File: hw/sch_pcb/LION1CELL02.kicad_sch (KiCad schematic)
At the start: 82 parts, among them IC1 BQ294602DRVR, J1 CONN1_1, J10 JUMP_2x1, J11 JUMP_2x1, J12 JUMP_2x1, J13 JUMP_2x1, J2 CONN1_1, J3 Jack-DC, J4 JUMP_2x1, J5 JUMP_2x1, J6 JUMP_2x1, J7 JUMP_2x1, J8 JUMP2_2x1, J9 Conn_02x03_Odd_Even, M1 HOLE M3, M2 HOLE M3, M3 HOLE, M4 HOLE, Q1 IRLML6244, SW1 SW_PUSH, U1 BQ24103, U2 SN74HC164D, U3 BQ34Z100

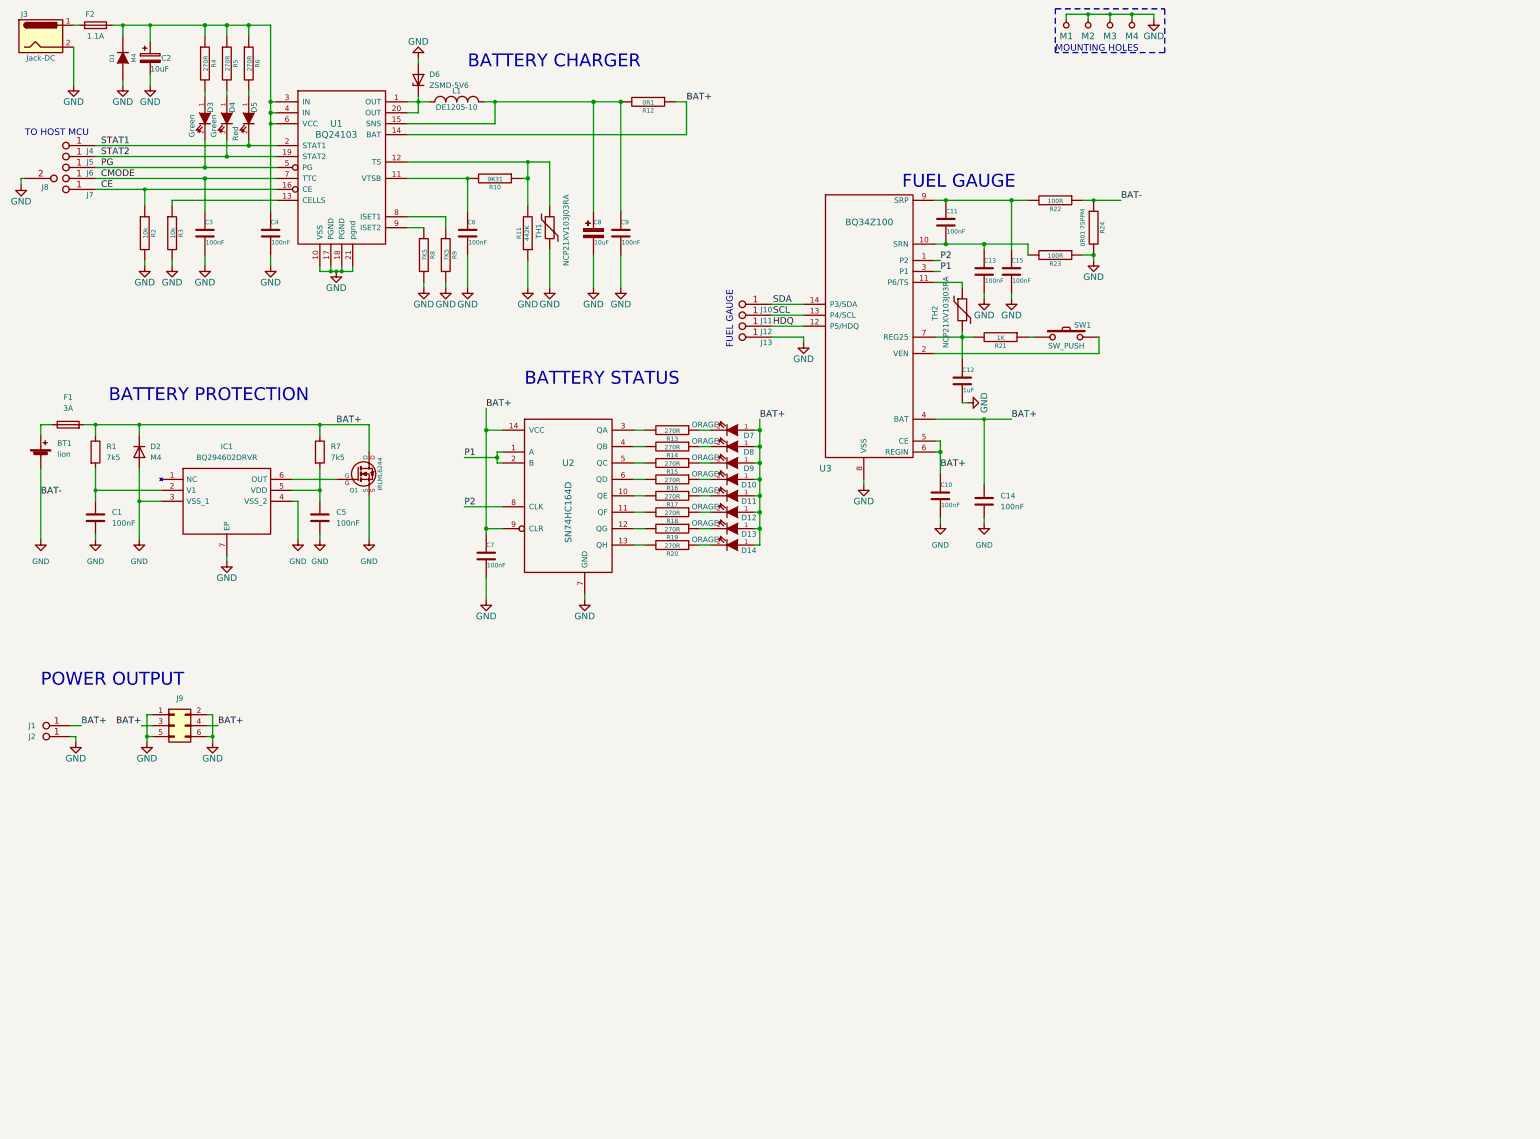
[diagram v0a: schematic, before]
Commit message: Update schematics
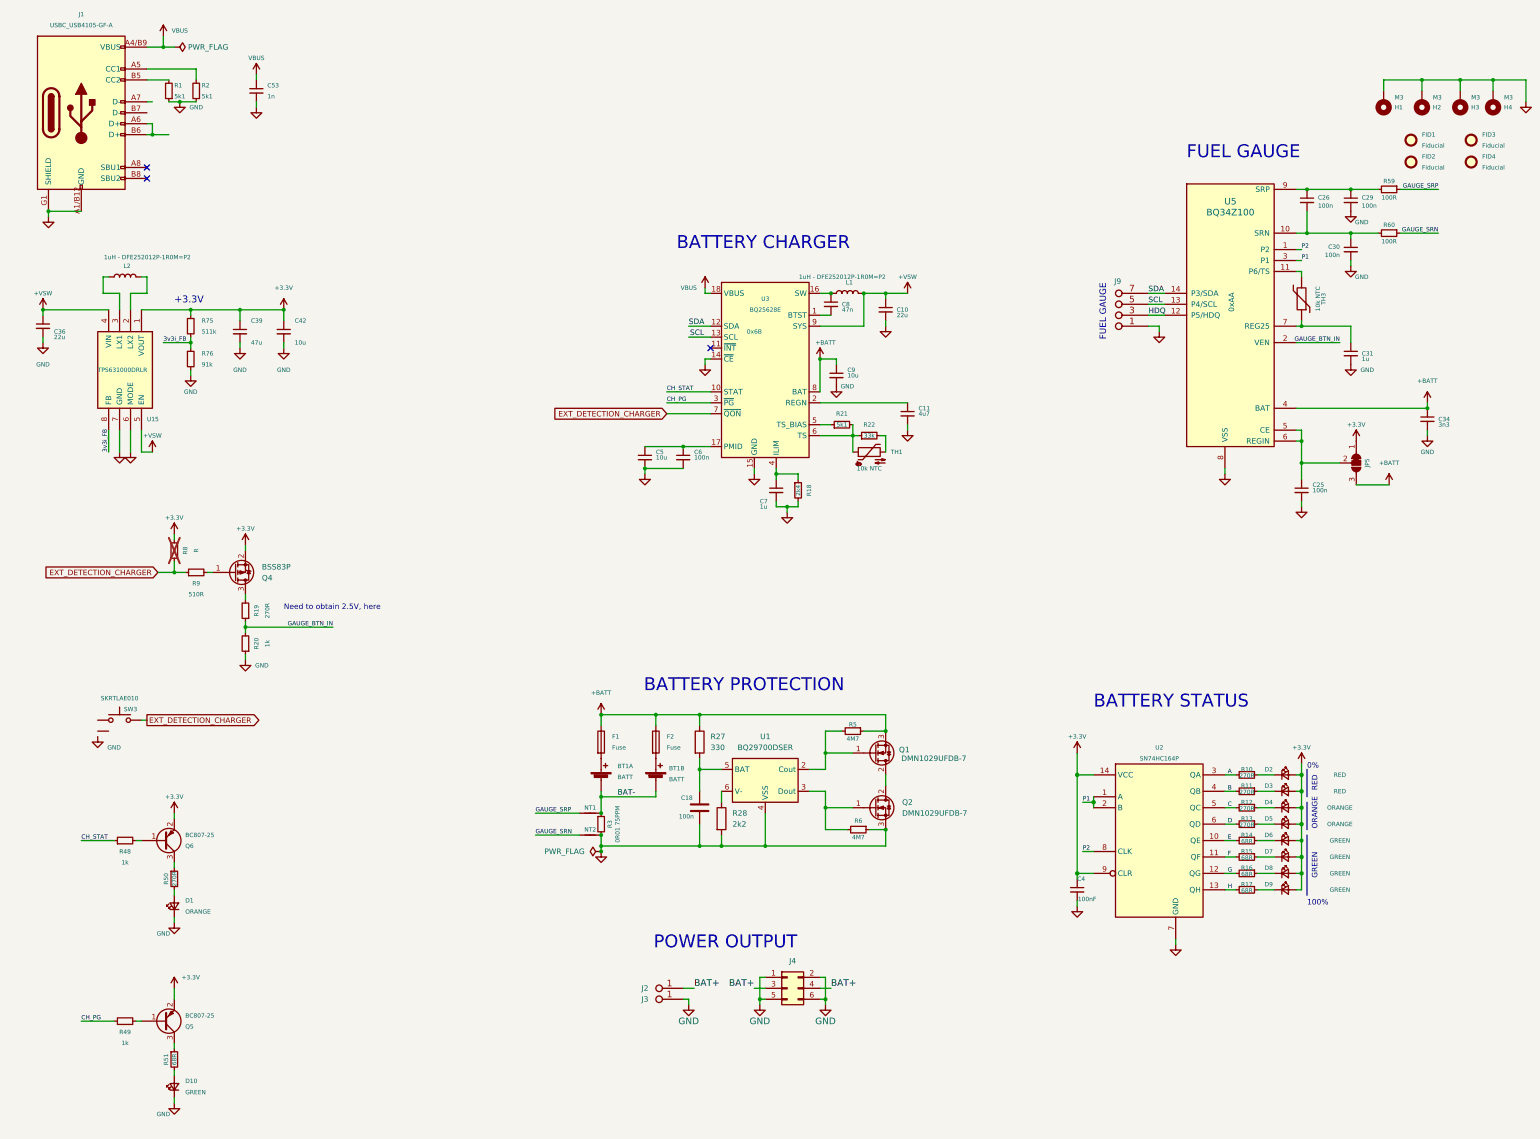
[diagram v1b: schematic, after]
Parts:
- removed BT1: lion, symbol Device:Battery_Cell
- removed C1, C14, C5: 100nF, Mlab_C:SMD-0805, symbol Device:C
- removed C10, C11, C13, C3, C4, C6, C7, C9: 100nF, Mlab_C:SMD-0805, symbol LION2CELL01D-rescue:C-RESCUE-LION2CELL01C
- removed C12: 1uF, Mlab_C:SMD-0805, symbol LION2CELL01D-rescue:C-RESCUE-LION2CELL01C
- removed C15: 100nF, Mlab_R:SMD-0805, symbol LION2CELL01D-rescue:C-RESCUE-LION2CELL01C
- removed C2: 10uF, Mlab_C:TantalC_SizeD_Reflow, symbol Device:C_Polarized
- removed C8: 10uF, Mlab_C:TantalC_SizeD_Reflow, symbol LION2CELL01D-rescue:CP2
- removed D1: M4, Mlab_D:SMA_Standard, symbol LION2CELL01D-rescue:DIODE
- removed D10, D11, D12, D13, D14, D7, D8, D9: ORAGE, Mlab_D:LED_1206, symbol LION2CELL01D-rescue:LED-RESCUE-LION2CELL01C
- removed D2: M4, symbol Device:D
- removed D3, D4: Green, Mlab_D:LED_1206, symbol LION2CELL01D-rescue:LED-RESCUE-LION2CELL01C
- removed D5: Red, Mlab_D:LED_1206, symbol LION2CELL01D-rescue:LED-RESCUE-LION2CELL01C
- removed D6: ZSMD-5V6, symbol Device:D_Zener
- removed IC1: BQ294602DRVR, symbol BQ294602DRVR:BQ294602DRVR
- removed J10, J11, J12, J13, J4, J5, J6, J7: JUMP_2x1, Mlab_Pin_Headers:Straight_1x02, symbol LION2CELL01D-rescue:JUMP_2x1
- removed J3: Jack-DC, symbol Connector:Jack-DC
- removed J8: JUMP2_2x1, symbol LION2CELL01D-rescue:JUMP2_2x1
- removed L1: DE1205-10, Mlab_L:DE1205-10, symbol LION2CELL01D-rescue:INDUCTOR_SMALL
- removed M1, M2: HOLE M3, Mlab_Mechanical:MountingHole_3mm, symbol mlab-default-rescue:HOLE
- removed M3, M4: HOLE, Mlab_Mechanical:MountingHole_3mm, symbol mlab-default-rescue:HOLE
- removed Q1: IRLML6244, Mlab_T:SOT-23, symbol LION2CELL01D-rescue:MOSFET-N
- removed R1, R7: 7k5, symbol Device:R
- removed R10: 9K31, Mlab_R:SMD-0805, symbol LION2CELL01D-rescue:R-RESCUE-LION2CELL01C
- removed R11: 442K, Mlab_R:SMD-0805, symbol LION2CELL01D-rescue:R-RESCUE-LION2CELL01C
- removed R12: 0R1, Resistors_SMD:R_2512, symbol LION2CELL01D-rescue:R-RESCUE-LION2CELL01C
- removed R13, R14, R15, R16, R17, R18, R19, R20, R4, R5, R6: 270R, Mlab_R:SMD-0805, symbol LION2CELL01D-rescue:R-RESCUE-LION2CELL01C
- removed R2, R3: 10k, Mlab_R:SMD-0805, symbol LION2CELL01D-rescue:R-RESCUE-LION2CELL01C
- removed R21: 1K, Mlab_R:SMD-0805, symbol LION2CELL01D-rescue:R-RESCUE-LION2CELL01C
- removed R22, R23: 100R, Mlab_R:SMD-0805, symbol LION2CELL01D-rescue:R-RESCUE-LION2CELL01C
- removed R24: 0R01 75PPM, Mlab_R:SMD-2512, symbol LION2CELL01D-rescue:R-RESCUE-LION2CELL01C
- removed R8, R9: 7K5, Mlab_R:SMD-0805, symbol LION2CELL01D-rescue:R-RESCUE-LION2CELL01C
- removed SW1: SW_PUSH, Mlab_SW:SW_PUSH_SMALL, symbol LION2CELL01D-rescue:SW_PUSH
- removed TH1, TH2: NCP21XV103J03RA, symbol Device:Thermistor
- removed U1: BQ24103, Mlab_IO:VQFN-20, symbol LION2CELL01D-rescue:BQ24103
- removed U2: SN74HC164D, Mlab_IO:SO-14, symbol LION2CELL01D-rescue:SN74HC164D
- removed U3: BQ34Z100, Mlab_IO:TSSOP-14_4.4x5mm_Pitch0.65mm, symbol LION2CELL01D-rescue:BQ34Z100
- added BT1: BATT, Mlab_Batery:BAT_BK-18650-PC4, symbol MLAB_BATERY:2xBATT
- added C10, C36: 22u, Capacitor_SMD:C_0805_2012Metric, symbol Device:C_Small
- added C11: 4u7, Capacitor_SMD:C_0805_2012Metric, symbol Device:C_Small
- added C18: 100n, symbol Device:C
- added C25, C26, C29, C30, C6: 100n, Capacitor_SMD:C_0805_2012Metric, symbol Device:C_Small
- added C31, C7: 1u, Capacitor_SMD:C_0805_2012Metric, symbol Device:C_Small
- added C34: 3n3, Capacitor_SMD:C_0805_2012Metric, symbol Device:C_Small
- added C39: 47u, Capacitor_SMD:C_0805_2012Metric, symbol Device:C_Small
- added C4: 100nF, Capacitor_SMD:C_0805_2012Metric, symbol Device:C_Small
- added C42, C5, C9: 10u, Capacitor_SMD:C_0805_2012Metric, symbol Device:C_Small
- added C53: 1n, Capacitor_SMD:C_0805_2012Metric, symbol Device:C_Small
- added C8: 47n, Capacitor_SMD:C_0805_2012Metric, symbol Device:C_Small
- added D1, D4, D5: ORANGE, Mlab_D:SMD_LED_RIGHT_KINGBRIGHT_1605, symbol Device:LED_Small
- added D10, D6, D7, D8, D9: GREEN, Mlab_D:SMD_LED_RIGHT_KINGBRIGHT_1605, symbol Device:LED_Small
- added D2, D3: RED, Mlab_D:SMD_LED_RIGHT_KINGBRIGHT_1605, symbol Device:LED_Small
- added FID1, FID2, FID3, FID4: Fiducial, Fiducial:Fiducial_1mm_Mask2mm, symbol Mechanical:Fiducial
- added H1, H2, H3, H4: M3, Mlab_Mechanical:MountingHole_3mm, symbol Mechanical:MountingHole_Pad
- added J1: USBC_USB4105-GF-A, Mlab_CON:USBC GCT_USB4105-GF-A, symbol MLAB_CONNECTORS:USBC_USB4105-GF-A
- added J9: JUMP_4X2, symbol MLAB_Jumpers:JUMP_4X2
- added JP5: Jumper_3_Bridged12, Jumper:SolderJumper-3_P1.3mm_Bridged2Bar12_RoundedPad1.0x1.5mm, symbol Jumper:SolderJumper_3_Bridged12
- added L1, L2: 1uH - DFE252012P-1R0M=P2, Inductor_SMD:L_1008_2520Metric, symbol Device:L
- added NT1, NT2: NetTie_2, NetTie:NetTie-2_SMD_Pad0.5mm, symbol Device:NetTie_2
- added Q1, Q2: DMN1029UFDB-7, symbol Transistor_FET:Q_NMOS_GDS
- added Q4: BSS83P, Package_TO_SOT_SMD:SOT-23, symbol Device:Q_PMOS_GSD
- added Q5, Q6: BC807-25, Package_TO_SOT_SMD:SOT-23-3, symbol Device:Q_PNP_BEC
- added R1, R2, R21: 5k1, Resistor_SMD:R_0805_2012Metric, symbol Device:R_Small
- added R10, R11, R12, R13, R19, R50: 270R, Resistor_SMD:R_0805_2012Metric, symbol Device:R_Small
- added R14, R15, R16, R17, R51: 68R, Resistor_SMD:R_0805_2012Metric, symbol Device:R_Small
- added R18: 2k4, Resistor_SMD:R_0805_2012Metric, symbol Device:R_Small
- added R20, R48, R49: 1k, Resistor_SMD:R_0805_2012Metric, symbol Device:R_Small
- added R22: 33k, Resistor_SMD:R_0805_2012Metric, symbol Device:R_Small
- added R27: 330, symbol Device:R
- added R28: 2k2, symbol Device:R
- added R3: 0R01 75PPM, Resistor_SMD:R_2512_6332Metric, symbol Device:R_Small
- added R5, R6: 4M7, Resistor_SMD:R_0805_2012Metric, symbol Device:R_Small
- added R59, R60: 100R, Resistor_SMD:R_0805_2012Metric, symbol Device:R_Small
- added R75: 511k, Resistor_SMD:R_0805_2012Metric, symbol Device:R_Small
- added R76: 91k, Resistor_SMD:R_0805_2012Metric, symbol Device:R_Small
- added R8: R, Resistor_SMD:R_0805_2012Metric, symbol Device:R_Small
- added R9: 510R, Resistor_SMD:R_0805_2012Metric, symbol Device:R_Small
- added SW3: SKRTLAE010, Mlab_SW:SKRT, symbol MLAB_SW:SW_Push_shield
- added TH1: 10k NTC, Resistor_SMD:R_0805_2012Metric, symbol Device:Thermistor_NTC
- added TH3: 10k NTC, Resistor_SMD:R_0805_2012Metric, symbol Device:Thermistor
- added U1: BQ29700DSER, Package_SON:WSON-6_1.5x1.5mm_P0.5mm, symbol Battery_Management:BQ297xy
- added U15: TPS631000DRLR, Package_TO_SOT_SMD:SOT-583-8, symbol MLAB_U:TPS631000DRLR
- added U2: SN74HC164P, Package_SO:TSSOP-14_4.4x5mm_P0.65mm, symbol MLAB_IO:SN74HC164D
- added U3: BQ25628E, Mlab_IO:Texas_S-WQFN-HR-18, symbol MLAB_IO:BQ25628E
- added U5: BQ34Z100, Mlab_IO:TSSOP-14_4.4x5mm_Pitch0.65mm, symbol MLAB_IO:BQ34Z100
- F1: value 3A -> Fuse; footprint (none) -> Fuse:Fuseholder_Littelfuse_Nano2_154x; UST_ID (none) -> 5c70984512875079b91f88d8
- F2: value 1.1A -> Fuse; footprint (none) -> Fuse:Fuseholder_Littelfuse_Nano2_154x; UST_ID (none) -> 5c70984512875079b91f88d8
- renumbered J1 to J2, J2 to J3, J9 to J4
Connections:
- net BAT+: no longer F1.2
- net GND: now also C10.2, C11.2, C18.2, C25.2, C29.2, C30.2, C31.2, C34.2, C36.2, C39.2, C4.2, C42.2, C5.2, C53.2, C6.2, C7.2, C9.2, D1.1 (K), D10.1 (K), H1.1, H2.1, H3.1, H4.1, J1.A1/B12 (GND), J1.B1/A12 (GND), J1.G1 (SHIELD), J1.G2 (SHIELD), J1.G3 (SHIELD), J1.G4 (SHIELD), J9.1 (2), J9.2, NT2.2, Q2.3 (S), R1.1, R18.2, R2.1, R20.1, R28.2, R3.2, R6.1, R76.2, U1.4 (VSS), U15.6 (MODE), U15.7 (GND), U2.7 (GND), U3.14 (~{CE}), U3.15 (GND), U5.8 (VSS)
- net HDQ: now also J9.3 (4), J9.4, U5.12 (P5/HDQ)
- net P1: now also U2.1 (A), U2.2 (B), U5.3 (P1)
- net P2: now also U2.8 (CLK), U5.1 (P2)
- net SCL: now also J9.5, J9.6 (5), U3.13 (SCL), U5.13 (P4/SCL)
- net SDA: now also J9.7 (8), J9.8, U3.12 (SDA), U5.14 (P3/SDA)
- net at F2.2: now also BT1.2+ (+)
- net +BATT: now reaches F2.1
- net +BATT: now also F1.1, C34.1, C9.1, JP5.3 (B), Q1.3 (S), R27.1, R5.1, U3.8 (BAT), U5.4 (BAT)
- new net: J1.B5 (CC2), R1.2
- new net: D6.1 (K), R14.1
- new net: C26.2, C30.1, R60.2, U5.10 (SRN)
- new net: Q5.3 (C), R51.1
- new net: D10.2 (A), R51.2
- new net: D7.1 (K), R15.1
- new net: BT1.1+ (+), F1.2
- new net: Q5.1 (B), R49.2
- new net: C25.1, JP5.2 (C), U5.5 (CE), U5.6 (REGIN)
- new net: D9.1 (K), R17.1
- new net: C7.1, R18.1, U3.4 (ILIM)
- new net: L2.1, U15.3 (LX1)
- new net: L2.2, U15.2 (LX2)
- new net: C8.1, L1.1, U3.16 (SW)
- new net: C8.2, U3.1 (BTST)
- new net: C26.1, C29.1, R59.2, U5.9 (SRP)
- new net: R21.1, U3.5 (TS_BIAS)
- new net: R21.2, R22.1, TH1.1, U3.6 (TS)
- new net: Q2.1 (G), R6.2, U1.3 (Dout)
- new net: C31.1, TH3.1, U5.7 (REG25)
- new net: Q1.1 (G), R5.2, U1.2 (Cout)
- new net: Q1.2 (D), Q2.2 (D)
- new net: Q6.1 (B), R48.2
- new net: TH3.2, U5.11 (P6/TS)
- new net: Q4.1 (G), R9.2
- new net: Q4.3 (D), R19.2
- new net: D5.1 (K), R13.1
- new net: C18.1, R27.2, U1.5 (BAT)
- new net: D4.1 (K), R12.1
- new net: D2.1 (K), R10.1
- new net: R28.1, U1.6 (V-)
- new net: J1.A5 (CC1), R2.2
- new net: R22.2, TH1.2
- new net: D3.1 (K), R11.1
- new net: C5.1, C6.1, U3.17 (PMID)
- new net: C11.1, U3.2 (REGN)
- new net: D1.2 (A), R50.2
- new net: J1.A6 (D+), J1.B6 (D+)
- new net: D8.1 (K), R16.1
- new net: Q6.3 (C), R50.1
- new net +3.3V: C39.1, C4.1, C42.1, D2.2 (A), D3.2 (A), D4.2 (A), D5.2 (A), D6.2 (A), D7.2 (A), D8.2 (A), D9.2 (A), JP5.1 (A), Q4.2 (S), Q5.2 (E), Q6.2 (E), R75.1, R8.2, U15.1 (VOUT), U2.14 (VCC), U2.9 (CLR)
- new net +VSW: C10.1, C36.1, L1.2, U15.4 (VIN), U15.5 (EN), U3.9 (SYS)
- new net 3v3i_FB: R75.2, R76.1, U15.8 (FB)
- new net A: R10.2, U2.3 (QA)
- new net B: R11.2, U2.4 (QB)
- new net BAT-: BT1.1- (-), BT1.2- (-), NT1.2, R3.1
- new net C: R12.2, U2.5 (QC)
- new net CH_PG: R49.1, U3.3 (~{PG})
- new net CH_STAT: R48.1, U3.10 (STAT)
- new net D: R13.2, U2.6 (QD)
- new net E: R14.2, U2.10 (QE)
- new net EXT_DETECTION_CHARGER: R8.1, R9.1, SW3.1, U3.7 (~{QON})
- new net F: R15.2, U2.11 (QF)
- new net G: R16.2, U2.12 (QG)
- new net GAUGE_BTN_IN: R19.1, R20.2, U5.2 (VEN)
- new net GAUGE_SRN: NT2.1, R60.1
- new net GAUGE_SRP: NT1.1, R59.1
- new net H: R17.2, U2.13 (QH)
- new net VBUS: C53.1, J1.A4/B9 (VBUS), J1.B4/A9 (VBUS), U3.18 (VBUS)
- no-connect marks 0 -> 3
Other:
- note added: "+3.3V"
- note added: "0%"
- note added: "100%"
- note added: "GREEN"
- note added: "Need to obtain 2.5V, here"
- note added: "ORANGE"
- note added: "RED"
- note removed: "MOUNTING HOLES"
- note removed: "TO HOST MCU"
- moved on the sheet: J2, J3, J4

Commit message: Update schematics
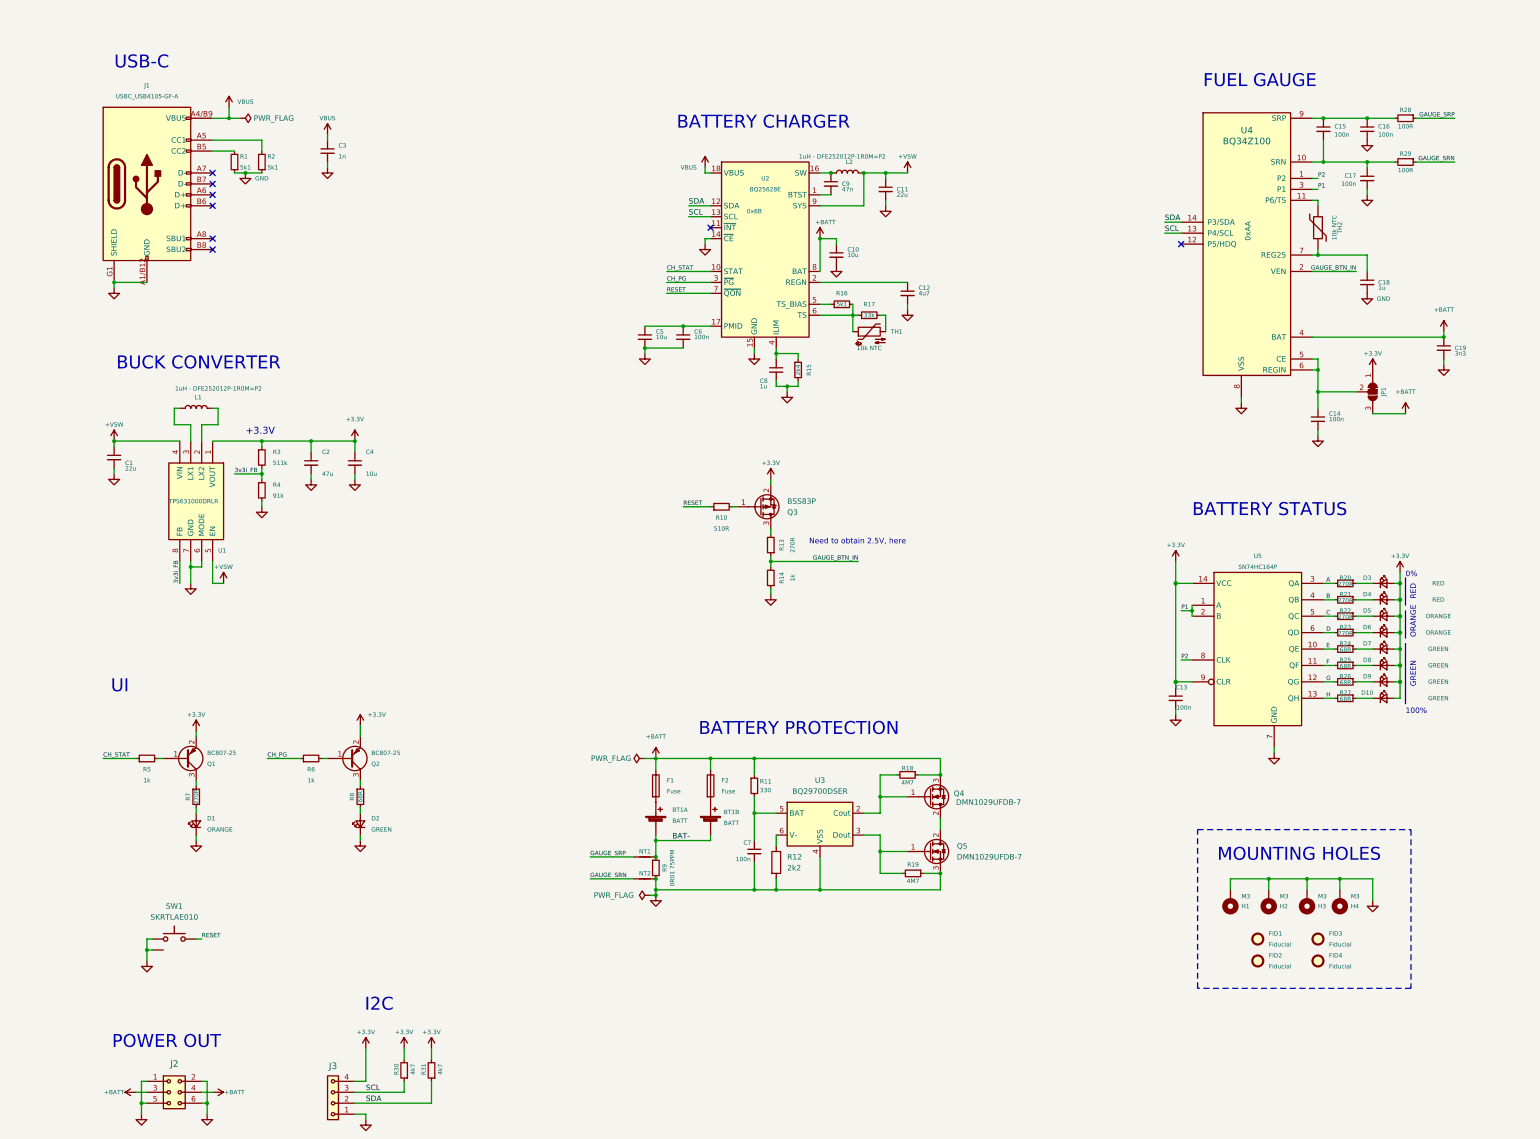
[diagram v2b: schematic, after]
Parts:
- removed C18: 100n, symbol Device:C
- removed J2, J3: CONN1_1, Mlab_Con:WAGO256, symbol LION2CELL01D-rescue:CONN1_1
- removed J4: Conn_02x03_Odd_Even, symbol Connector_Generic:Conn_02x03_Odd_Even
- removed J9: JUMP_4X2, symbol MLAB_Jumpers:JUMP_4X2
- removed R27: 330, symbol Device:R
- removed R8: R, Resistor_SMD:R_0805_2012Metric, symbol Device:R_Small
- removed SW3: SKRTLAE010, Mlab_SW:SKRT, symbol MLAB_SW:SW_Push_shield
- added C7: 100n, Capacitor_SMD:C_0805_2012Metric, symbol Device:C_Small
- added J2: HEADER_2x03, Connector_PinHeader_2.54mm:PinHeader_2x03_P2.54mm_Vertical, symbol MLAB_HEADER:HEADER_2x03
- added J3: HEADER_1x04, Connector_PinHeader_2.54mm:PinHeader_1x04_P2.54mm_Horizontal, symbol MLAB_HEADER:HEADER_1x04
- added R11: 330, symbol Device:R_Small
- added R30, R31: 4k7, Resistor_SMD:R_0805_2012Metric, symbol Device:R_Small
- added SW1: SKRTLAE010, Mlab_SW:SKRT, symbol MLAB_SW:SW_Push_shield
- C13: renamed from C4; value 100nF -> 100n
- R12: renamed from R28; footprint (none) -> Resistor_SMD:R_0805_2012Metric
- renumbered C36 to C1, C9 to C10, C10 to C11, C11 to C12, C25 to C14, C26 to C15, C29 to C16, C30 to C17, C31 to C18, C34 to C19, C39 to C2, C53 to C3, C42 to C4, C7 to C8, C8 to C9, D9 to D10, D10 to D2, D2 to D3, D3 to D4, D4 to D5, D5 to D6, D6 to D7, D7 to D8, D8 to D9, JP5 to JP1, L2 to L1, L1 to L2, Q6 to Q1, Q5 to Q2, Q4 to Q3, Q1 to Q4, Q2 to Q5, R9 to R10, R19 to R13, R20 to R14, R18 to R15, R21 to R16, R22 to R17, R5 to R18, R6 to R19, R10 to R20, R11 to R21, R12 to R22, R13 to R23, R14 to R24, R15 to R25, R16 to R26, R17 to R27, R59 to R28, R60 to R29, R75 to R3, R76 to R4, R48 to R5, R49 to R6, R50 to R7, R51 to R8, R3 to R9, TH3 to TH2, U15 to U1, U3 to U2, U1 to U3, U5 to U4, U2 to U5
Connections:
- net +3.3V: now also J3.4, R30.2, R31.2
- net +BATT: now also J2.3, J2.4, R11.1
- net GND: now also C7.2, J2.1, J2.2, J2.5, J2.6, J3.1, SW1.2, SW1.GND (SHIELD)
- net SCL: now also J3.3, R30.1
- net SDA: now also J3.2, R31.1
- net at U3.5 (BAT): now also C7.1, R11.2
- net at J1.A6 (D+): no longer J1.B6 (D+)
- net EXT_DETECTION_CHARGER renamed RESET
- net RESET: now also SW1.1
- net HDQ: no longer names the net of U4.12 (P5/HDQ)
- no-connect marks 3 -> 8
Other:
- note added: "BUCK CONVERTER"
- note added: "I2C"
- note added: "MOUNTING HOLES"
- note added: "POWER OUT"
- note added: "UI"
- note added: "USB-C"
- note removed: "POWER OUTPUT"
- moved on the sheet: BT1A, BT1B, C1, C10, C11, C12, C13, C14, C15, C16, C17, C18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

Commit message: Repository cleanup.
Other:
- company: Mlab.cz -> MLAB.cz
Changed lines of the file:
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@@
 		(title "LION1CELL02A")
 		(date "2024-07-17")
-		(company "Mlab.cz")
+		(company "MLAB.cz")
 		(comment 1 "Singe cell Li-ion battery management\\nwith USB-C charger")
 	)
